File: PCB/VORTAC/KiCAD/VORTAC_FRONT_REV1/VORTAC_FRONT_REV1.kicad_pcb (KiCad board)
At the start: 4 copper layers, 31.7 x 51.3 mm, 6 parts, among them J1 Conn_02x02_Odd_Even, J2 Conn_02x03_Odd_Even, J3 Conn_01x07

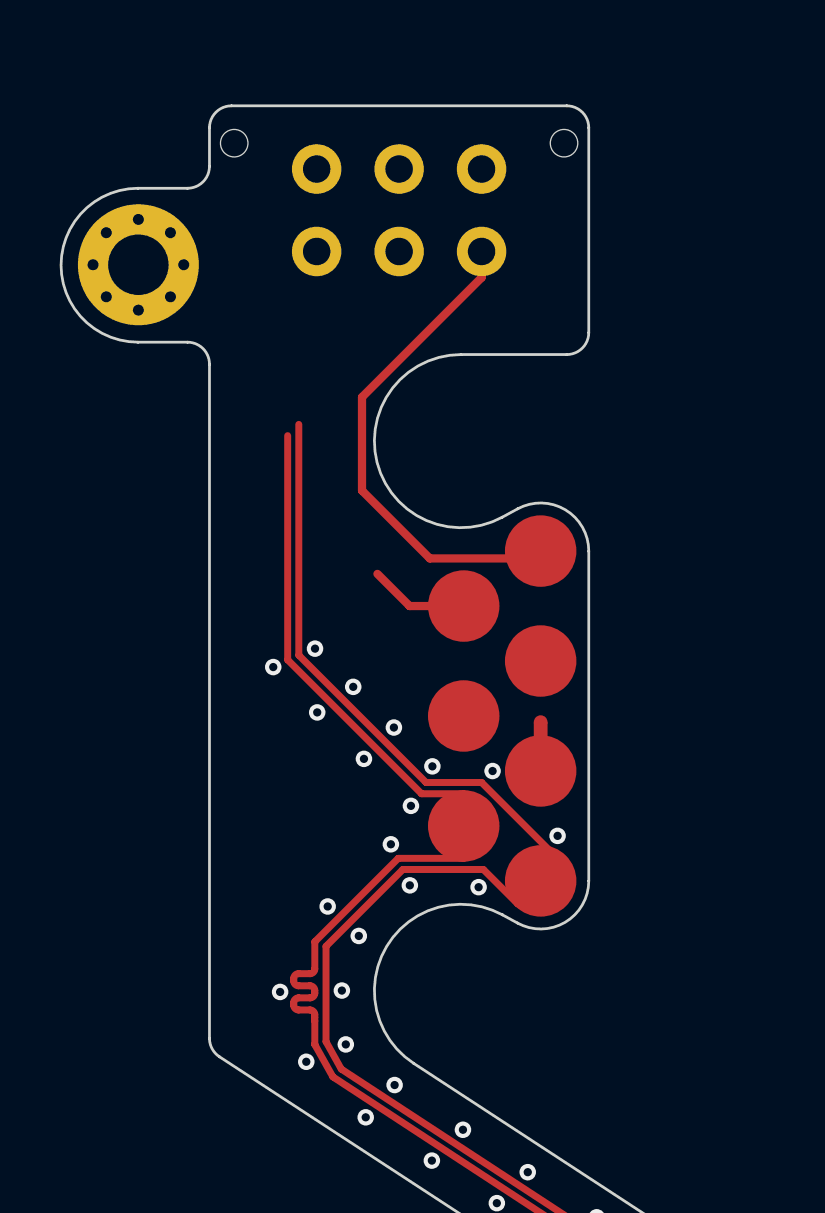
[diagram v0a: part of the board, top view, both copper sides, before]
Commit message: Churro
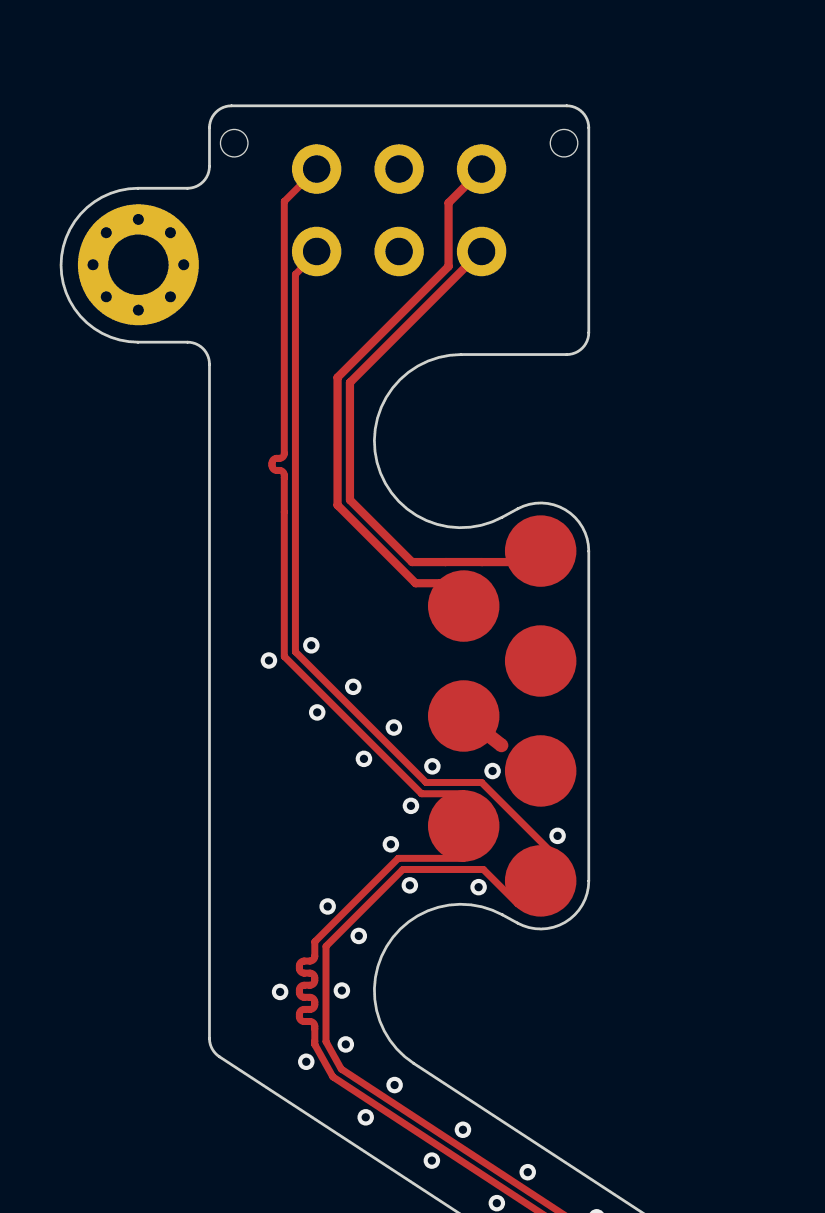
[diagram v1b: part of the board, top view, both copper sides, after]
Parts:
- moved NT1 1.82 mm to (111.1, 79.4), turned to -38 degrees
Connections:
- J2 pad 1: CAN_L -> CAN_H
- J2 pad 4: CAN_H -> CAN_L
- J3 pad 3: GND -> VDC
- J3 pad 4: VDC -> TOOL_ID
- J3 pad 5: TOOL_ID -> GND
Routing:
- net USB_D-: track 3.62 -> 20.5 mm
- net CAN_L: track 50.1 -> 60.9 mm
- net CAN_H: track 54.5 -> 61.2 mm
- net USB_D+: track 17.2 -> 18.1 mm

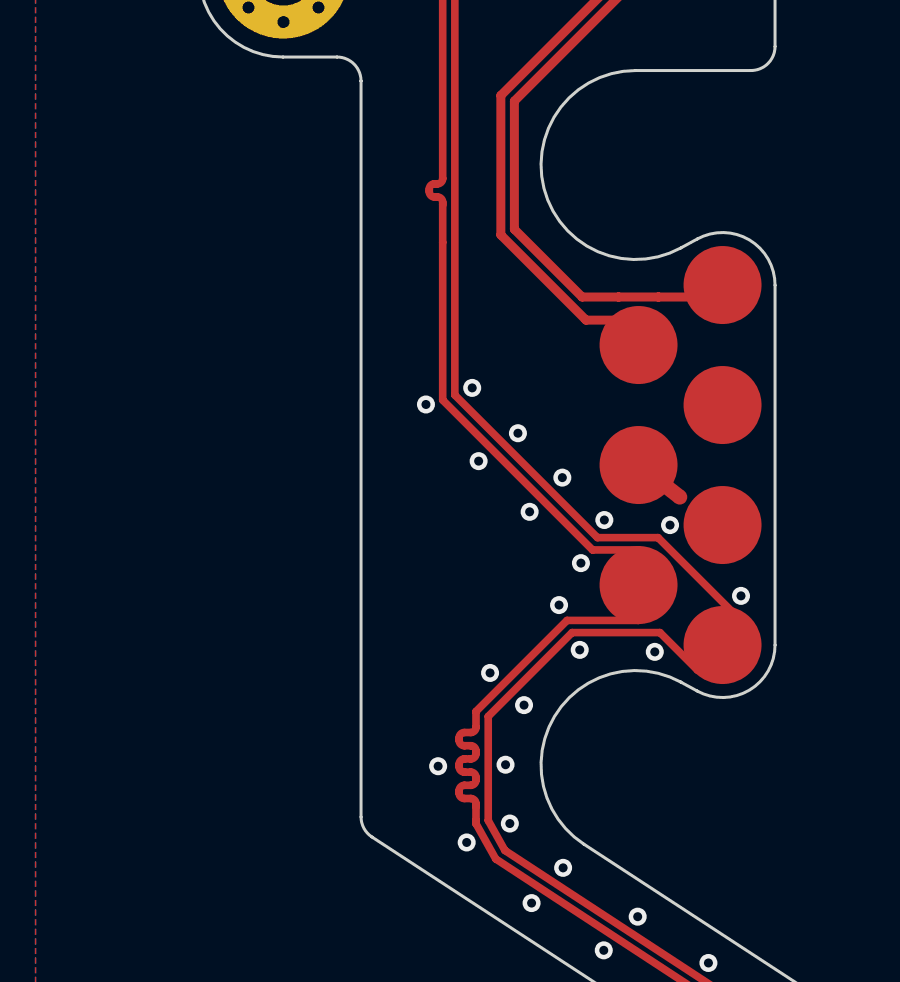
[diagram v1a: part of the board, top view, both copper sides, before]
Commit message: KONGSTRONG
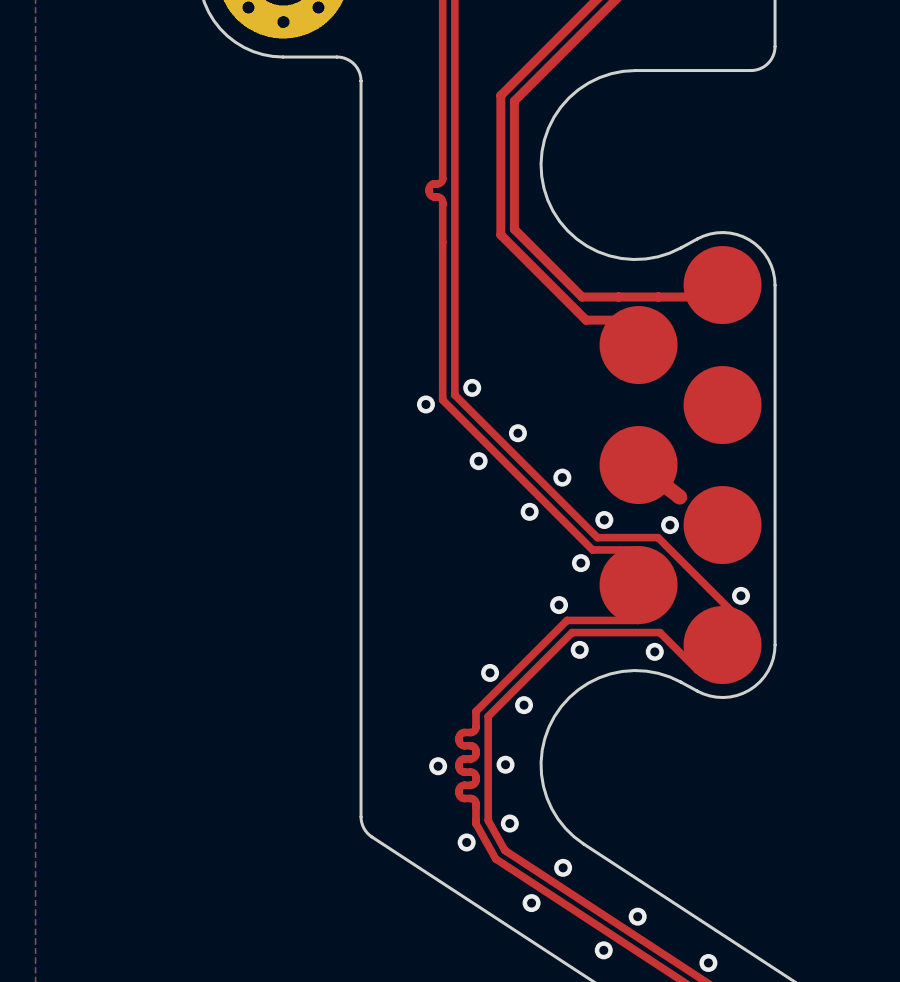
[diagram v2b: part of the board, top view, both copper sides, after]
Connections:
- J2 pad 2: GND -> VDC
- J2 pad 5: VDC -> GND
